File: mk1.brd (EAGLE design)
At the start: 114.3 x 76.2 mm, 28 parts, among them U1 IAM-20380, U2 MC34063AD, U3 ADXL345, U4 STM32F407VGT6

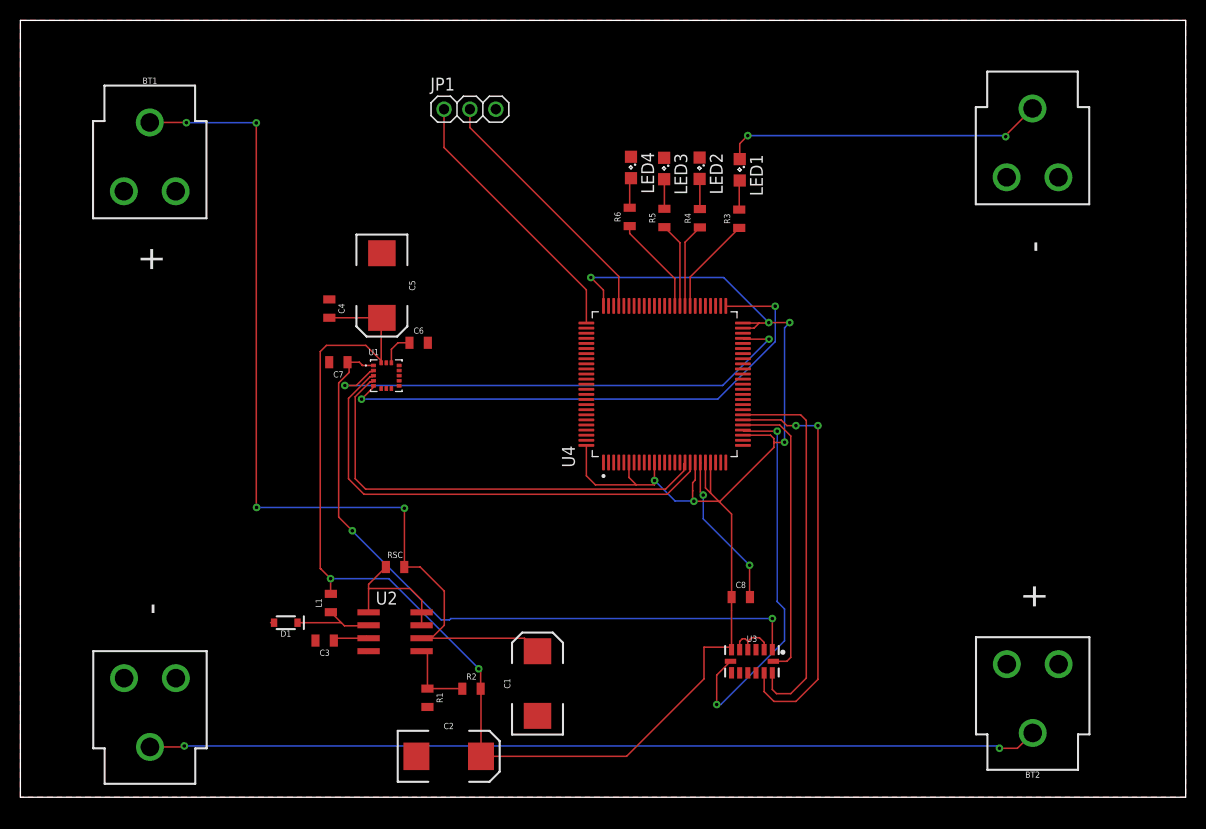
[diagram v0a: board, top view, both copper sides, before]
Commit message: Update Rev 1 with reroute
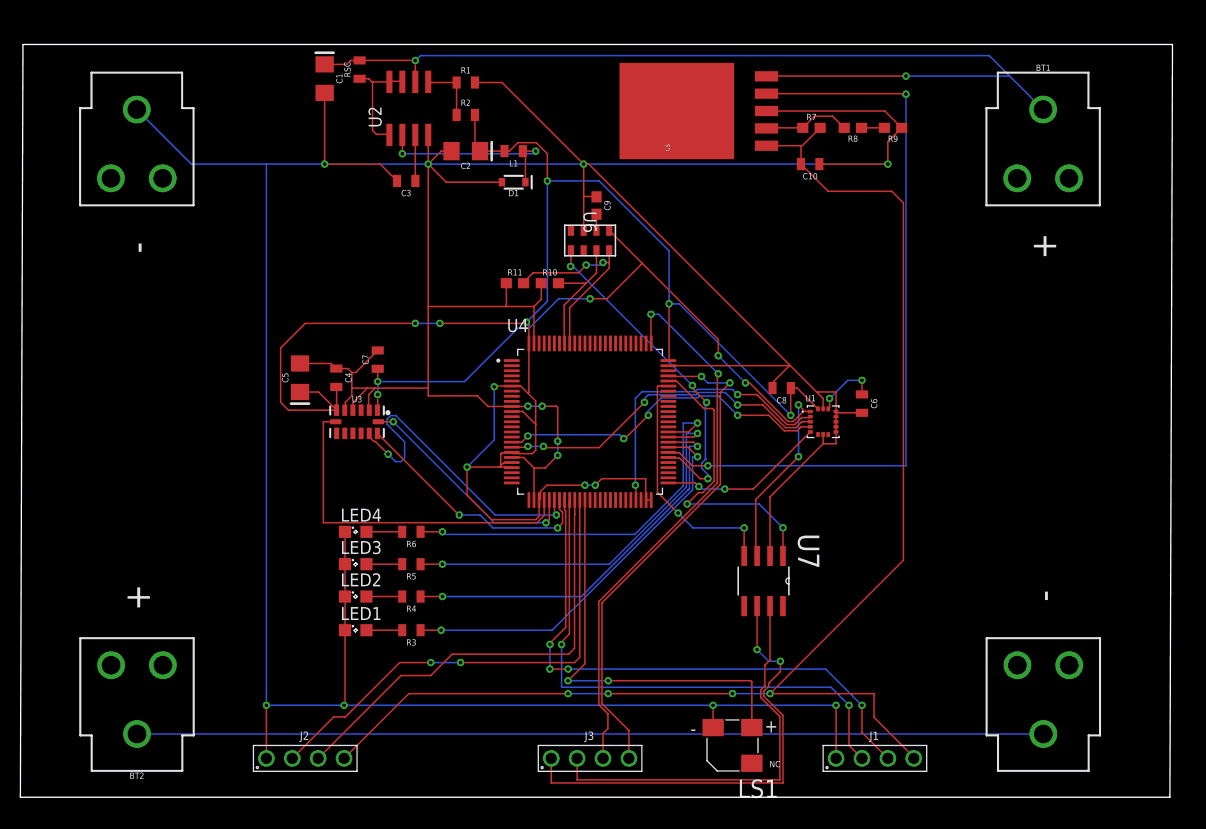
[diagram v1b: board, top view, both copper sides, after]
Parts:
- removed JP1: (no value), adafruit:1X03
- added C10: 22uF, SparkFun-Capacitors:0805
- added C9: 0.1uF, SparkFun-Capacitors:0603
- added J1, J2, J3: (no value), Wurth_Elektronik_Electromechanic_Board_to_Board_Connectors_rev18b:61300411121
- added LS1: CSS-0575A-SMT, CSS-0575A-SMT:CUI_CSS-0575A-SMT
- added R10, R11: 4.7k, SparkFun-Resistors:0603
- added R7: 200k, SparkFun-Resistors:0603
- added R8: 220k, SparkFun-Resistors:0603
- added R9: 43k, SparkFun-Resistors:0603
- added U5: LT1529CQTRPBF, LT1529CQTRPBF:DDPAK-5_Q
- added U6: MPL115A2, MPL115A2:LGA8
- added U7: SN65HVD232DR, SN65HVD232DR:SOIC127P600X175-8N
- C1: device SparkFun-Capacitors:EIA7343 -> SparkFun-Capacitors:1206-POLAR
- C2: value 50000uf -> 100uF; device SparkFun-Capacitors:EIA7343 -> SparkFun-Capacitors:1206-POLAR
- C5: value 2.2uf -> 100uF; device SparkFun-Capacitors:EIA7343 -> SparkFun-Capacitors:1206-POLAR
- L1: value 50uh -> 47uh
- moved BT2 87.9 mm to (11.4, 36.8)
- moved BT1 87.6 mm to (100.3, 36.8)
- moved C1 62.9 mm to (29.8, 70.5), turned to 270 degrees
- moved R1 60.5 mm to (43.7, 70.1), turned to 0 degrees
- moved C2 59.4 mm to (43.7, 63.4), turned to 180 degrees
- moved LED1 58.8 mm to (32.9, 16.4), turned to 0 degrees
- moved R2 56.3 mm to (43.7, 66.9)
- moved LED2 53.9 mm to (32.9, 19.7), turned to 0 degrees
- moved R3 51.6 mm to (38.4, 16.4), turned to 180 degrees
- moved U2 51.4 mm to (38.1, 67.6), turned to 0 degrees
- moved LED3 49.2 mm to (32.9, 22.9), turned to 0 degrees
- moved RSC 48.9 mm to (33.3, 71.4), turned to 90 degrees
- moved D1 48.6 mm to (48.4, 60.3)
- moved L1 47.8 mm to (48.4, 63.4), turned to 180 degrees
- moved R4 46.7 mm to (38.4, 19.7), turned to 180 degrees
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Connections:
- removed net N$15: JP1.2, U4.72
- removed net N$16: JP1.1, U4.76
- removed net N$6: C7.1, U1.1, U3.1
- new net +3V3: C7.1, U1.1, U3.1, U6.1, U7.3
- new net BENABLE: U4.56, U6.5
- new net BSCL: R11.2, U4.92, U6.8
- new net BSDA: R10.2, U4.93, U6.7
- new net BSHD: U6.4
- new net BUZZER: LS1.1, U4.37
- new net CANH: J3.2, U7.7
- new net CANL: J3.1, U7.6
- new net CANRX: U4.70, U7.4
- new net CANTX: U4.71, U7.1
- new net JTCK: J3.3, U4.76
- new net N$18: R7.1, R8.2, U5.2
- new net N$19: R8.1, R9.2
- new net N$22: C9.2, U6.2
- new net S1IN: J1.2, U4.34
- new net S1O: J1.3, U4.33
- new net S2IN: J2.2, U4.36
- new net S2O: J2.3, U4.35
- new net SERVOPWR: U4.57, U5.4
- new net SWDIO: J3.4, U4.72
- new net V7+: C10.2, J1.4, J2.4, R7.2, U5.1
- net 3.3V: now also C2.1, C5.1; no longer C2.A, C5.A
- net BATIN: now also C1.1, U5.5; no longer C1.A
- net GND: now also C1.2, C10.1, C2.2, C5.2, C9.1, J1.1, J2.1, LS1.2, R10.1, R11.1, R9.1, U5.3, U6.3, U7.2; no longer C1.C, C2.C, C5.C
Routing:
- net GND: track 53.1 -> 457.1 mm, vias 4 -> 12
- net V7+: track 0.00 -> 135.3 mm, vias 0 -> 4
- net +3V3: track 0.00 -> 81.1 mm, vias 0 -> 7
- net SERVOPWR: track 0.00 -> 73.9 mm, vias 0 -> 2
- net N$6: track 68.2 -> 0.00 mm, vias 2 -> 0
- net S1O: track 0.00 -> 55.7 mm, vias 0 -> 4
- net JTCK: track 0.00 -> 54.8 mm, vias 0 -> 2
- net S1IN: track 0.00 -> 53.1 mm, vias 0 -> 2
- net SWDIO: track 0.00 -> 49.4 mm, vias 0 -> 2
- net S2IN: track 0.00 -> 47.7 mm, vias 0 -> 2
- net CANL: track 0.00 -> 45.6 mm, vias 0 -> 2
- net S2O: track 0.00 -> 44.2 mm
- net BUZZER: track 0.00 -> 40.9 mm, vias 0 -> 2
- net CANH: track 0.00 -> 40.2 mm
- net SSG: track 53.0 -> 16.5 mm
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- removed copper zone on layer 1, net GND
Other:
- board size 114.3 x 76.2 mm -> 113 x 73.8 mm
- board text added: "Rocket Mk 1.0 Rev 1.0 Robert Murphy & Dawson Moore"
